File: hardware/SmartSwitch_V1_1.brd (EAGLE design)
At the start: 49 x 49 mm, 46 parts, among them K1 FTR-LYC5, K2 FTR-LYC5, U2 AMS1117-3.3

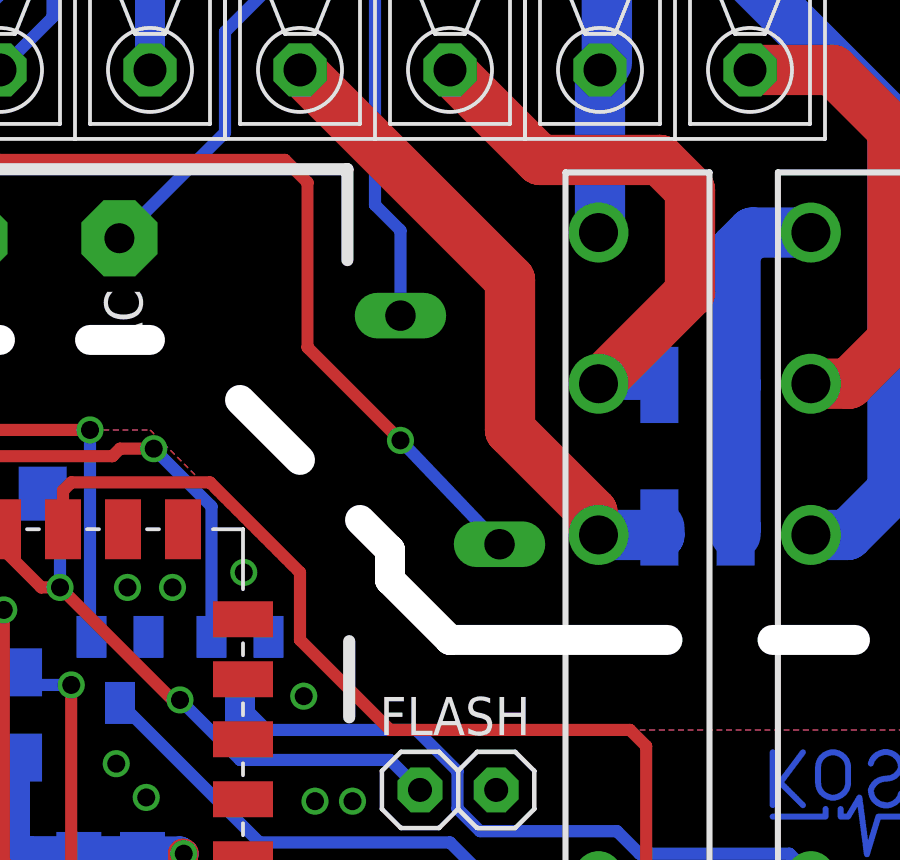
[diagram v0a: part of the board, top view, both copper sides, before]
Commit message: Add files via upload
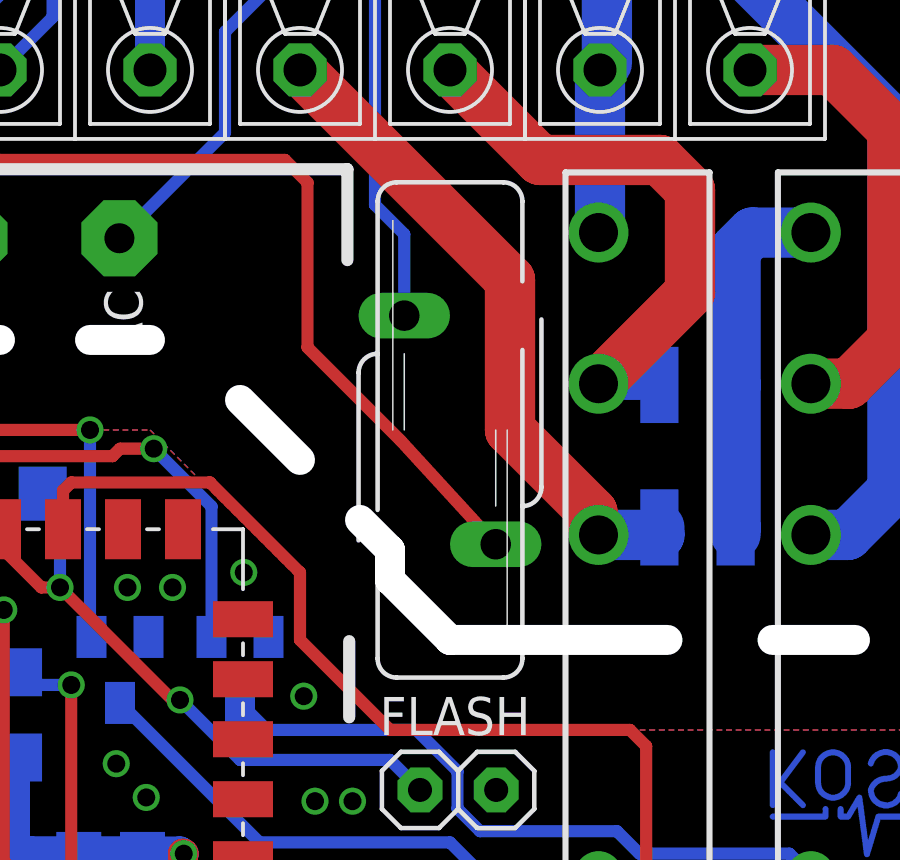
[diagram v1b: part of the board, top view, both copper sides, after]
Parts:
- R7: value S14K275 -> S14K275GESPIEGELT; device varistor:S14K275 -> varistor:S14K275_
- flipped R7 to the top
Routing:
- net HV.N: track 48.8 -> 48.7 mm, vias 1 -> 0
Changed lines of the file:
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@@
 <?xml version="1.0" encoding="utf-8"?>
 <!DOCTYPE eagle SYSTEM "eagle.dtd">
-<eagle version="7.2.0">
+<eagle version="6.2">
 <drawing>
 <settings>
@@
 <grid distance="1" unitdist="mm" unit="mm" style="lines" multiple="1" display="yes" altdistance="0.125" altunitdist="mm" altunit="mm"/>
 <layers>
-<layer number="1" name="Top" color="4" fill="1" visible="no" active="yes"/>
-<layer number="16" name="Bottom" color="1" fill="1" visible="yes" active="yes"/>
+<layer number="1" name="Top" color="17" fill="1" visible="yes" active="yes"/>
+<layer number="16" name="Bottom" color="16" fill="1" visible="yes" active="yes"/>
 <layer number="17" name="Pads" color="2" fill="1" visible="yes" active="yes"/>
 <layer number="18" name="Vias" color="2" fill="1" visible="yes" active="yes"/>
 <layer number="19" name="Unrouted" color="13" fill="1" visible="yes" active="yes"/>
 <layer number="20" name="Dimension" color="15" fill="1" visible="yes" active="yes"/>
-<layer number="21" name="tPlace" color="7" fill="1" visible="no" active="yes"/>
-<layer number="22" name="bPlace" color="7" fill="1" visible="yes" active="yes"/>
+<layer number="21" name="tPlace" color="4" fill="1" visible="yes" active="yes"/>
+<layer number="22" name="bPlace" color="1" fill="1" visible="yes" active="yes"/>
 <layer number="23" name="tOrigins" color="15" fill="1" visible="yes" active="yes"/>
 <layer number="24" name="bOrigins" color="15" fill="1" visible="yes" active="yes"/>
 <layer number="25" name="tNames" color="7" fill="1" visible="no" active="yes"/>
-<layer number="26" name="bNames" color="7" fill="1" visible="yes" active="yes"/>
+<layer number="26" name="bNames" color="7" fill="1" visible="no" active="yes"/>
 <layer number="27" name="tValues" color="7" fill="1" visible="no" active="yes"/>
 <layer number="28" name="bValues" color="7" fill="1" visible="no" active="yes"/>
@@
 <layer number="49" name="Reference" color="7" fill="1" visible="no" active="yes"/>
 <layer number="50" name="dxf" color="7" fill="1" visible="no" active="no"/>
-<layer number="51" name="tDocu" color="7" fill="1" visible="yes" active="yes"/>
-<layer number="52" name="bDocu" color="7" fill="1" visible="yes" active="yes"/>
+<layer number="51" name="tDocu" color="7" fill="1" visible="no" active="yes"/>
+<layer number="52" name="bDocu" color="7" fill="1" visible="no" active="yes"/>
 <layer number="53" name="tGND_GNDA" color="7" fill="9" visible="no" active="no"/>
 <layer number="54" name="bGND_GNDA" color="1" fill="9" visible="no" active="no"/>
@@
 </class>
 </classes>
-<designrules name="default">
+<designrules>
 <description language="de">&lt;b&gt;EAGLE Design Rules&lt;/b&gt;
 &lt;p&gt;
@@
 <pass name="Default">
 <param name="RoutingGrid" value="50mil"/>
-<param name="AutoGrid" value="1"/>
-<param name="Efforts" value="0"/>
-<param name="TopRouterVariant" value="1"/>
 <param name="tpViaShape" value="round"/>
 <param name="PrefDir.1" value="|"/>
@@
 <attribute name="VALUE" x="17.54" y="19.27" size="1.27" layer="28" rot="MR270"/>
 </element>
-<element name="R7" library="varistor" package="S14K275" value="S14K275" x="32" y="26.5" smashed="yes" rot="MR0">
-<attribute name="VALUE" x="35.429" y="26.119" size="1.27" layer="28" ratio="10" rot="MR90"/>
+<element name="R7" library="varistor" package="S14K275_" value="S14K275GESPIEGELT" x="32" y="26.5" smashed="yes">
+<attribute name="VALUE" x="28.571" y="26.119" size="1.27" layer="27" ratio="10" rot="R90"/>
 </element>
 <element name="F1" library="fuse" package="SMD_FUSE_HOLDER" value="0,4A" x="25" y="43.5" smashed="yes" rot="MR180"/>
@@
 <wire x1="27.25" y1="34.75" x2="27.25" y2="29.25" width="0.4064" layer="1"/>
 <wire x1="27.25" y1="29.25" x2="30.349" y2="26.151" width="0.4064" layer="1"/>
-<wire x1="30.349" y1="26.151" x2="33.651" y2="22.69" width="0.4064" layer="16"/>
+<wire x1="30.349" y1="26.151" x2="33.524" y2="22.69" width="0.4064" layer="1"/>
 <contactref element="R2" pad="1"/>
 <contactref element="R4" pad="1"/>
@@
 <wire x1="18.75" y1="45.5" x2="18.75" y2="40.25" width="0.4064" layer="16"/>
 <wire x1="18.75" y1="40.25" x2="17" y2="38.5" width="0.4064" layer="16"/>
-<via x="30.349" y="26.151" extent="1-16" drill="0.6" shape="octagon"/>
 <wire x1="12.422" y1="46.5" x2="14.5" y2="46.5" width="0.4064" layer="16"/>
 <wire x1="14.5" y1="46.5" x2="15.078" y2="45.922" width="0.4064" layer="16"/>
@@
 <wire x1="28.19" y1="43.31" x2="28" y2="43.5" width="1" layer="16"/>
 <wire x1="28.19" y1="43.46" x2="28.19" y2="43.31" width="1" layer="16"/>
-<wire x1="29.5" y1="34" x2="30.349" y2="33.151" width="0.4064" layer="16"/>
-<wire x1="30.349" y1="33.151" x2="30.349" y2="30.31" width="0.4064" layer="16"/>
+<wire x1="29.5" y1="34" x2="30.476" y2="33.024" width="0.4064" layer="16"/>
+<wire x1="30.476" y1="33.024" x2="30.476" y2="30.31" width="0.4064" layer="16"/>
 </signal>
 <signal name="RESET">
